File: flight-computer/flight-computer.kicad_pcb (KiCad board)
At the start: 2 copper layers, 25.4 x 51.5 mm, 37 parts, among them J1 Conn_01x06_Pin, J2 Conn_01x06_Pin, J3 Power Connector, J4 Micro_SD_Card, J5 USB_C_Receptacle_USB2.0_16P, J6 Conn_01x02_Pin, Q1 DMN3404L, Q2 DMN3404L, U1 LMR51420X, U2 ESP32-S3-WROOM-1, U3 LSM6DSO32TR, U4 INA2180A1IDGKR

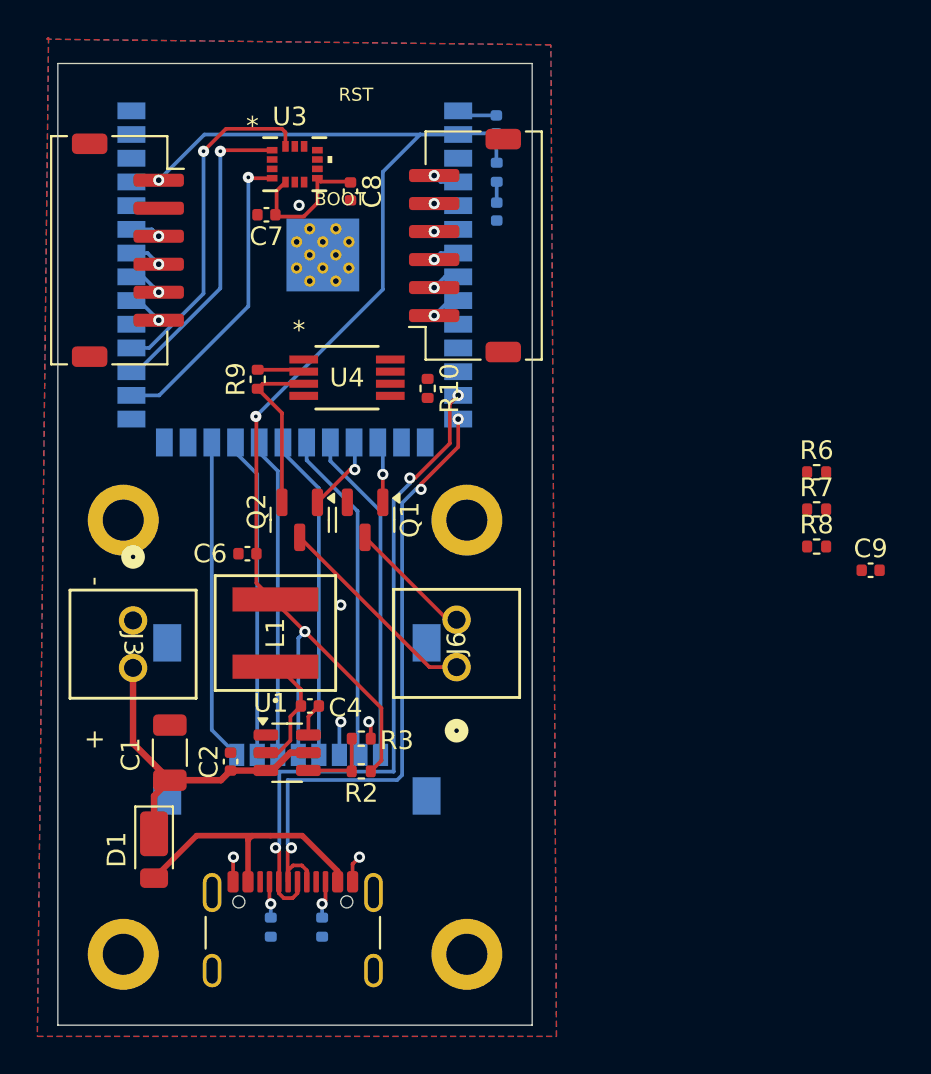
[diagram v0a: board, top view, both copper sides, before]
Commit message: finished connecting things
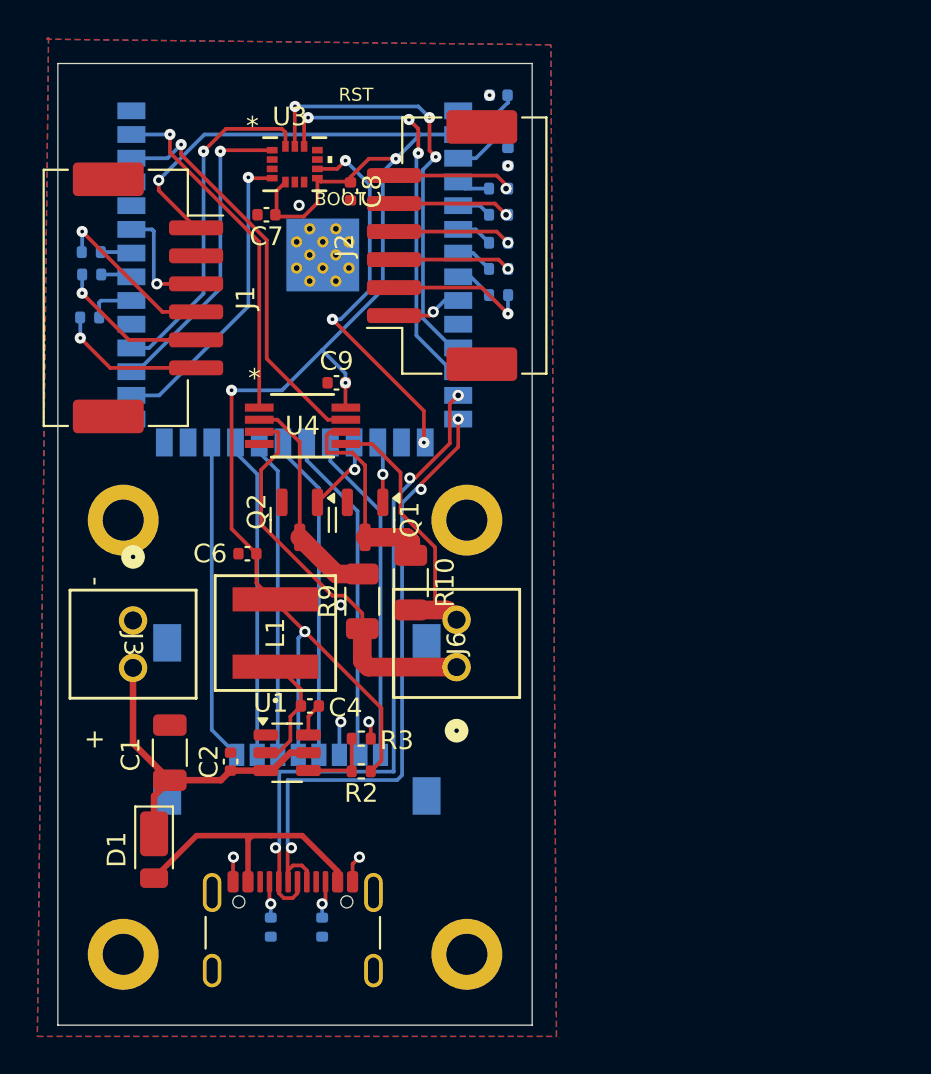
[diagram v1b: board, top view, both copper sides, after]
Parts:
- added R11: 200 Ohm, Resistor_SMD:R_0402_1005Metric, B.Cu at (133.9, 90.0)
- added R12: 200 Ohm, Resistor_SMD:R_0402_1005Metric, B.Cu at (155.7, 85.4)
- added R13: 200 Ohm, Resistor_SMD:R_0402_1005Metric, B.Cu at (155.7, 86.8)
- added R14: 200 Ohm, Resistor_SMD:R_0402_1005Metric, B.Cu at (155.7, 88.3)
- added R15: 200 Ohm, Resistor_SMD:R_0402_1005Metric, B.Cu at (155.7, 89.7)
- J1, J2: footprint Connector_JST:JST_ZH_S6B-ZR-SM4A-TF_1x06-1MP_P1.50mm_Horizontal -> Connector_JST:JST_ZE_SM06B-ZESS-TB_1x06-1MP_P1.50mm_Horizontal
- R10, R9: footprint Resistor_SMD:R_0402_1005Metric -> Resistor_SMD:R_1206_3216Metric
- R6, R7, R8: moved to B.Cu
- moved R7 41.2 mm to (133.9, 88.8)
- moved R6 39.8 mm to (133.8, 92.3)
- moved C9 30.3 mm to (147.0, 95.8)
- moved R8 21.7 mm to (155.7, 91.1), turned to 180 degrees
- moved R9 13.1 mm to (148.4, 107.5)
- moved R10 10.4 mm to (151.0, 106.5)
- moved U4 3.51 mm to (145.2, 98.1)
- moved C3 2.99 mm to (156.2, 83.7)
- moved J1 2.77 mm to (136.9, 91.3)
- moved R1 2.73 mm to (155.7, 81.8), turned to 0 degrees
- moved C5 1.56 mm to (155.7, 80.4), turned to 180 degrees
- moved J2 1.22 mm to (152.7, 88.5)
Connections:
- C9 pad 2: unconnected-(C9-Pad2) -> +3.3V
- J1 pad 5: FIN_MISO -> Net-(J1-Pin_5)
- J2 pad 3: FIN_CS4 -> Net-(J2-Pin_3)
- J2 pad 4: FIN_CS3 -> Net-(J2-Pin_4)
- J2 pad 5: FIN_CS2 -> Net-(J2-Pin_5)
- J2 pad 6: FIN_CS1 -> Net-(J2-Pin_6)
- Q1 pad 1: Net-(Q1-G) -> Remote Start 1
- Q1 pad 3: Net-(J6-Pin_2) -> Net-(Q1-D)
- Q2 pad 1: Net-(Q2-G) -> Remote Start 2
- Q2 pad 3: Net-(J6-Pin_1) -> Net-(Q2-D)
- R10 pad 1: Remote Start 1 -> Net-(Q1-D)
- R10 pad 2: Net-(Q1-G) -> Net-(J6-Pin_2)
- R9 pad 1: Net-(Q2-G) -> Net-(J6-Pin_1)
- R9 pad 2: Remote Start 2 -> Net-(Q2-D)
- U4 pad 2: Net-(Q2-G) -> Net-(Q2-D)
- U4 pad 3: Remote Start 2 -> Net-(J6-Pin_1)
- U4 pad 5: Remote Start 1 -> Net-(J6-Pin_2)
- U4 pad 6: Net-(Q1-G) -> Net-(Q1-D)
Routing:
- net LSM_SCK: track 0.00 -> 23.3 mm, vias 0 -> 3
- net LSM_CS: track 0.00 -> 22.0 mm, vias 0 -> 3
- net IMP_OUT2: track 0.00 -> 21.9 mm, vias 0 -> 1
- net LSM_INT2: track 0.00 -> 20.4 mm, vias 0 -> 3
- net IMP_OUT1: track 0.00 -> 18.8 mm, vias 0 -> 1
- net +3.3V: track 76.4 -> 88.8 mm, vias 3 -> 5
- net Net-(Q2-D): track 0.00 -> 11.9 mm
- net Net-(Q1-D): track 0.00 -> 11.5 mm
- net Net-(J6-Pin_1): track 11.3 -> 21.5 mm
- net (no net): track 9.19 -> 0.00 mm
- net Net-(J1-Pin_4): track 0.00 -> 8.99 mm, vias 0 -> 1
- net Net-(J1-Pin_5): track 0.00 -> 8.14 mm, vias 0 -> 1
- net Net-(J6-Pin_2): track 6.73 -> 14.8 mm
- net Net-(J1-Pin_6): track 0.00 -> 7.97 mm, vias 0 -> 1
- net Net-(J2-Pin_2): track 0.00 -> 7.68 mm, vias 0 -> 1
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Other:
- board text added: "ew please fix"
